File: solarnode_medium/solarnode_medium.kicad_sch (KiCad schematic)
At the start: 94 parts, among them J1 Conn_01x06, Q1 AO3400, Q2 AO3400, Q3 AO3400, Q4 Q_NMOS_GSD, SW1 3*4*2mm, U1 YX59012, U2 SGM2033-3.3, U3 MAX485E, U4 LM358, U5 SGM48211, U6 SGM48211, U7 YX59012

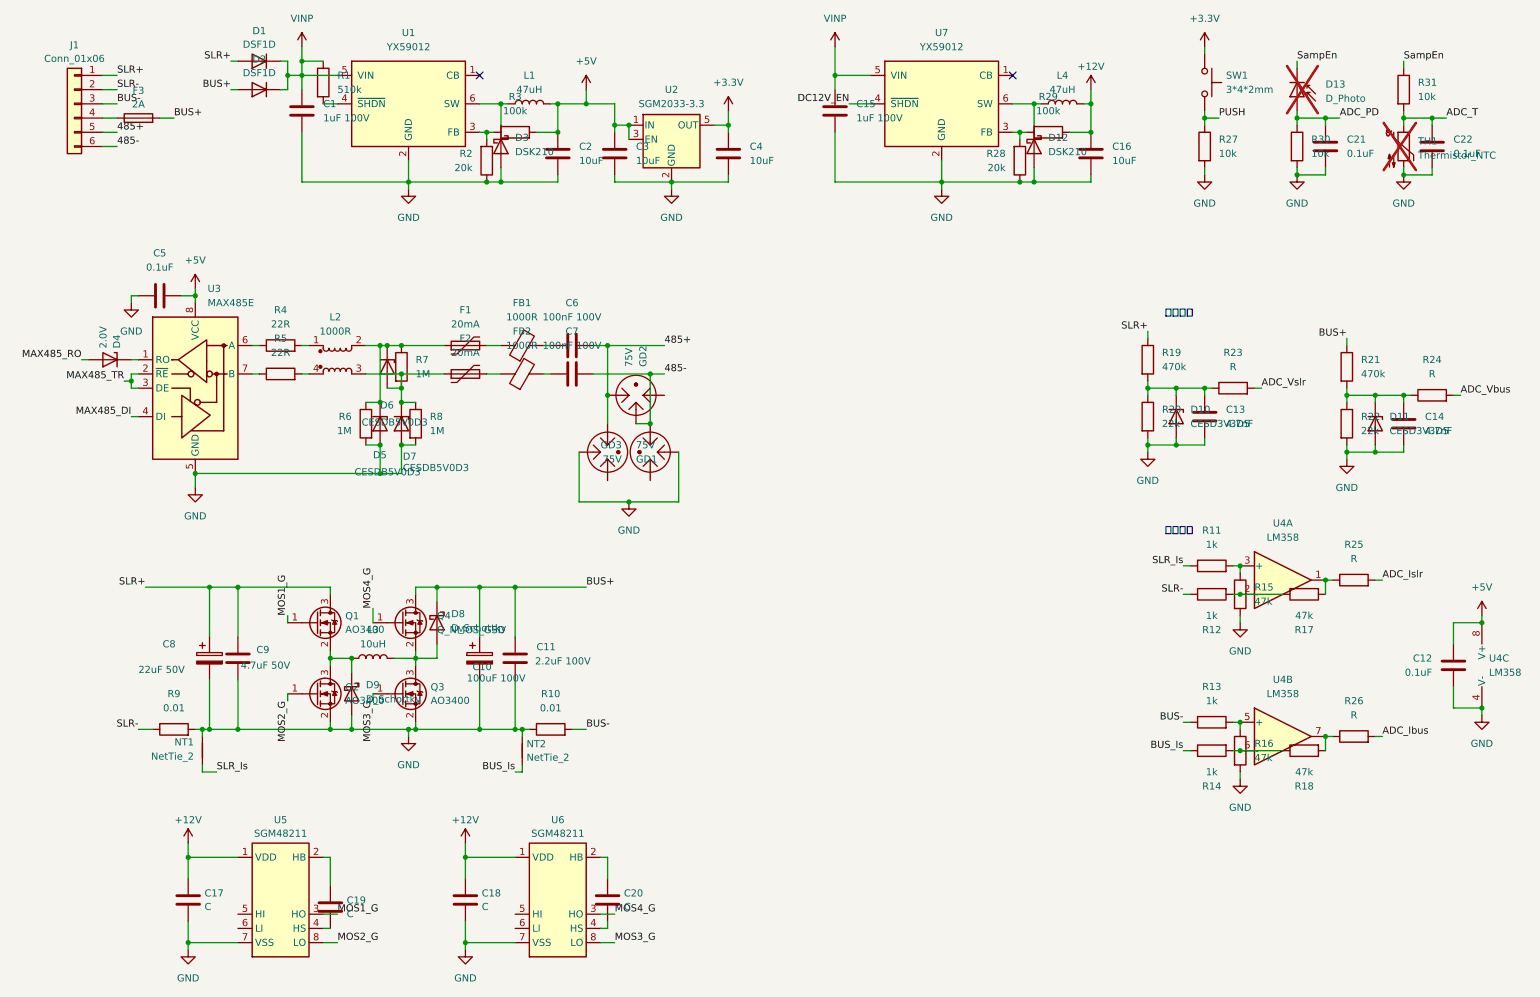
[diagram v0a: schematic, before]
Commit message: solarnode_medium划分子原理图
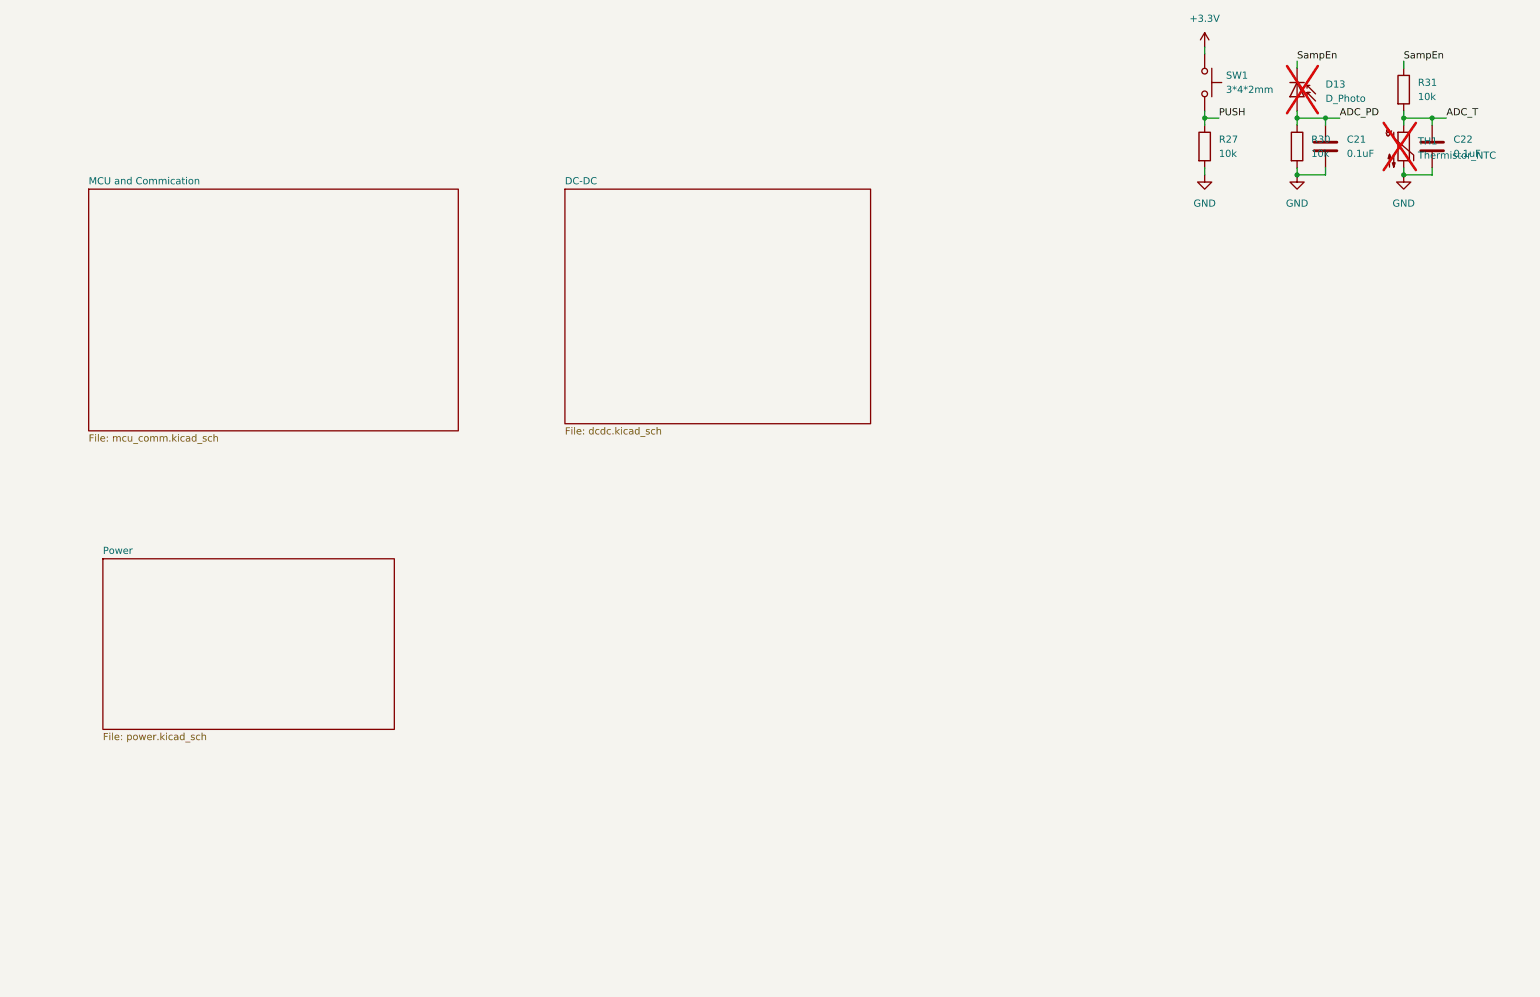
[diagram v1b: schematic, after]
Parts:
- removed C1, C15: 1uF 100V, Capacitor_SMD:C_0805_2012Metric, symbol Device:C
- removed C10: 100uF 100V, Capacitor_SMD:C_Elec_6.3x5.4, symbol Device:C_Polarized
- removed C11: 2.2uF 100V, Capacitor_SMD:C_1210_3225Metric, symbol Device:C
- removed C12: 0.1uF, Capacitor_SMD:C_0402_1005Metric, symbol Device:C
- removed C13, C14: 4.7nF, Capacitor_SMD:C_0402_1005Metric, symbol Device:C
- removed C16, C2, C3, C4: 10uF, Capacitor_SMD:C_0805_2012Metric, symbol Device:C
- removed C17, C18, C19, C20: C, symbol Device:C
- removed C5: 0.1uF, Capacitor_SMD:C_0603_1608Metric, symbol Device:C
- removed C6, C7: 100nF 100V, Capacitor_SMD:C_0603_1608Metric, symbol Device:C
- removed C8: 22uF 50V, Capacitor_SMD:C_Elec_6.3x5.4, symbol Device:C_Polarized
- removed C9: 4.7uF 50V, Capacitor_SMD:C_1210_3225Metric, symbol Device:C
- removed D1, D2: DSF1D, Diode_SMD:D_SOD-123F, symbol Device:D
- removed D10, D11: CESD3V3D5, Diode_SMD:D_SOD-523, symbol Device:D_Zener
- removed D12, D3: DSK210, Diode_SMD:D_SOD-123F, symbol Device:D_Schottky
- removed D4: 2.0V, Diode_SMD:D_SOD-323, symbol Device:D_Zener
- removed D5, D6, D7: CESDB5V0D3, Diode_SMD:D_SOD-323, symbol Diode:ESD5Zxx
- removed D8, D9: D_Schottky, symbol Device:D_Schottky
- removed F1, F2: 20mA, Fuse:Fuse_0603_1608Metric, symbol Device:Polyfuse
- removed F3: 2A, Fuse:Fuse_1206_3216Metric, symbol Device:Fuse
- removed FB1, FB2: 1000R, Inductor_SMD:L_0603_1608Metric, symbol Device:FerriteBead
- removed GD1, GD2, GD3: 75V, Capacitor_SMD:C_1206_3216Metric, symbol Device:GDT_3Pin
- removed J1: Conn_01x06, TerminalBlock:TerminalBlock_bornier-6_P5.08mm, symbol Connector_Generic:Conn_01x06
- removed L1, L4: 47uH, Inductor_SMD:L_1210_3225Metric, symbol Device:L
- removed L2: 1000R, Inductor_SMD:L_CommonModeChoke_Coilcraft_1812CAN, symbol Device:L_Coupled_1243
- removed L3: 10uH, Inductor_SMD:L_APV_APH0630, symbol Device:L
- removed NT1: NetTie_2, NetTie:NetTie-2_SMD_Pad0.5mm, symbol Device:NetTie_2
- removed NT2: NetTie_2, ProjectLibrary:NetTie-2_VIA_Pad0.6_0.3mm, symbol Device:NetTie_2
- removed Q1, Q2, Q3: AO3400, Package_TO_SOT_SMD:TO-252-2, symbol Device:Q_NMOS_GSD
- removed Q4: Q_NMOS_GSD, symbol Device:Q_NMOS_GSD
- removed R1: 510k, Resistor_SMD:R_0402_1005Metric, symbol Device:R
- removed R10, R9: 0.01, Resistor_SMD:R_1206_3216Metric, symbol Device:R
- removed R11, R12, R13, R14: 1k, Resistor_SMD:R_0402_1005Metric, symbol Device:R
- removed R15, R16, R17, R18: 47k, Resistor_SMD:R_0402_1005Metric, symbol Device:R
- removed R19, R21: 470k, Resistor_SMD:R_0603_1608Metric, symbol Device:R
- removed R2, R28: 20k, Resistor_SMD:R_0402_1005Metric, symbol Device:R
- removed R20, R22: 22k, Resistor_SMD:R_0402_1005Metric, symbol Device:R
- removed R23, R24, R25, R26: R, symbol Device:R
- removed R29, R3: 100k, Resistor_SMD:R_0402_1005Metric, symbol Device:R
- removed R4, R5: 22R, Resistor_SMD:R_0603_1608Metric, symbol Device:R
- removed R6, R7, R8: 1M, Resistor_SMD:R_0603_1608Metric, symbol Device:R
- removed U1, U7: YX59012, Package_TO_SOT_SMD:SOT-23-6, symbol Regulator_Switching:LV2862XDDC
- removed U2: SGM2033-3.3, Package_TO_SOT_SMD:SOT-23-5, symbol Regulator_Linear:TLV70033_SOT23-5
- removed U3: MAX485E, Package_SO:SOIC-8_3.9x4.9mm_P1.27mm, symbol Interface_UART:MAX485E
- removed U4: LM358, Package_SO:SOP-8_3.9x4.9mm_P1.27mm, symbol Amplifier_Operational:LM358
- removed U5, U6: SGM48211, Package_SO:SOIC-8_3.9x4.9mm_P1.27mm, symbol Driver_FET:HIP2100_SOIC
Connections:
- no-connect marks 2 -> 0
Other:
- added sheet DC-DC (dcdc.kicad_sch)
- added sheet MCU and Commication (mcu_comm.kicad_sch)
- added sheet Power (power.kicad_sch)
- note removed: "电压测量"
- note removed: "电流测量"
